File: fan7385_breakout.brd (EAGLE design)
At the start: 28.6 x 14 mm, 13 parts

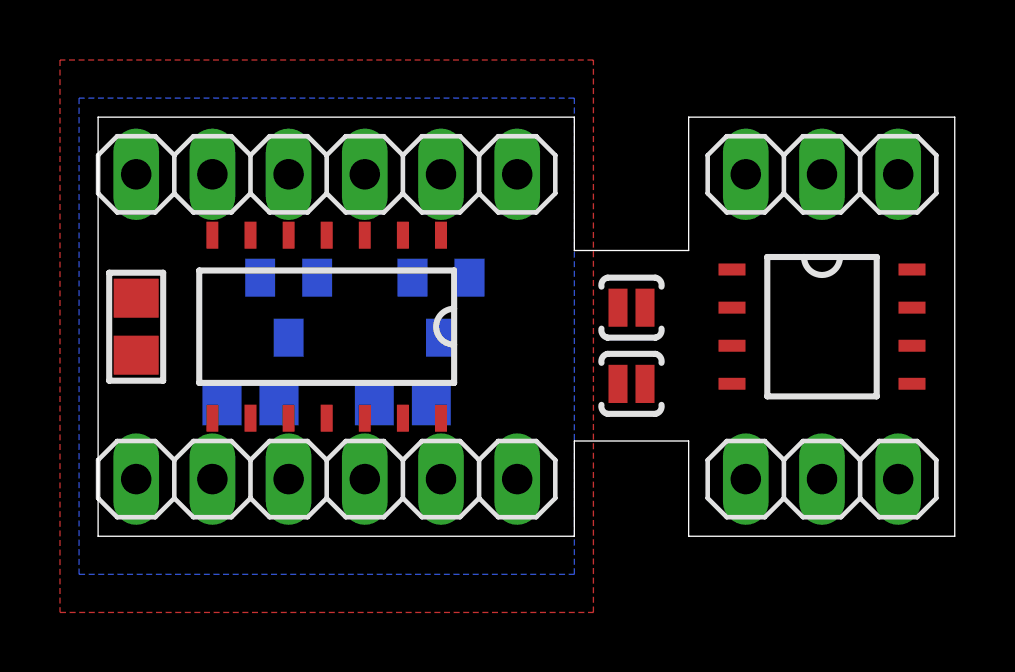
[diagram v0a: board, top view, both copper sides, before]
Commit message: autorouted
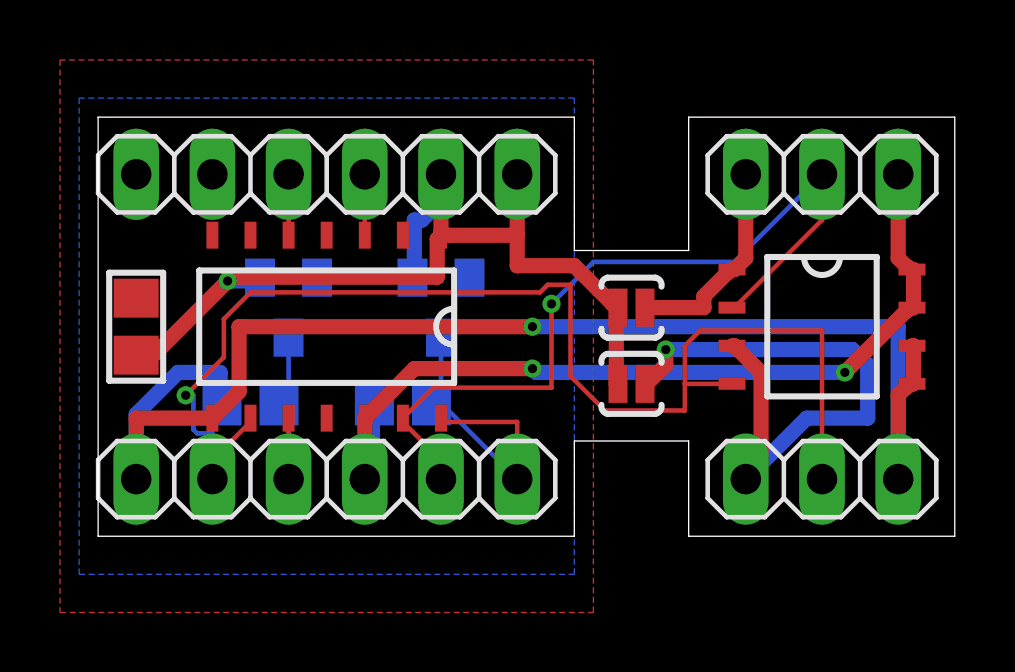
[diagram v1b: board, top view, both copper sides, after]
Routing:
- net D2/VS2: track 0.00 -> 46.4 mm, vias 0 -> 1
- net HO2/G2: track 0.00 -> 42.1 mm, vias 0 -> 1
- net VDD: track 0.00 -> 32.0 mm, vias 0 -> 1
- net D1/VS1: track 0.00 -> 29.5 mm, vias 0 -> 2
- net HO1/G1: track 0.00 -> 27.3 mm, vias 0 -> 1
- net S2: track 0.00 -> 20.2 mm, vias 0 -> 1
- net VB1: track 0.00 -> 11.0 mm
- net VB2: track 0.00 -> 7.38 mm
- net S1: track 0.00 -> 7.05 mm
- net IN2: track 0.00 -> 2.03 mm
- net IN1: track 0.00 -> 2.03 mm
